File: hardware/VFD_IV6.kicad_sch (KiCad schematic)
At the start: 94 parts, among them J1 Conn_01x09, Q2 BC817, U1 4511, U10 TBD62783A, U11 4511, U12 TBD62783A, U13 4017, U2 TBD62783A, U3 4511, U4 TBD62783A, U5 4511, U6 TBD62783A, U7 4511, U8 TBD62783A, U9 4511

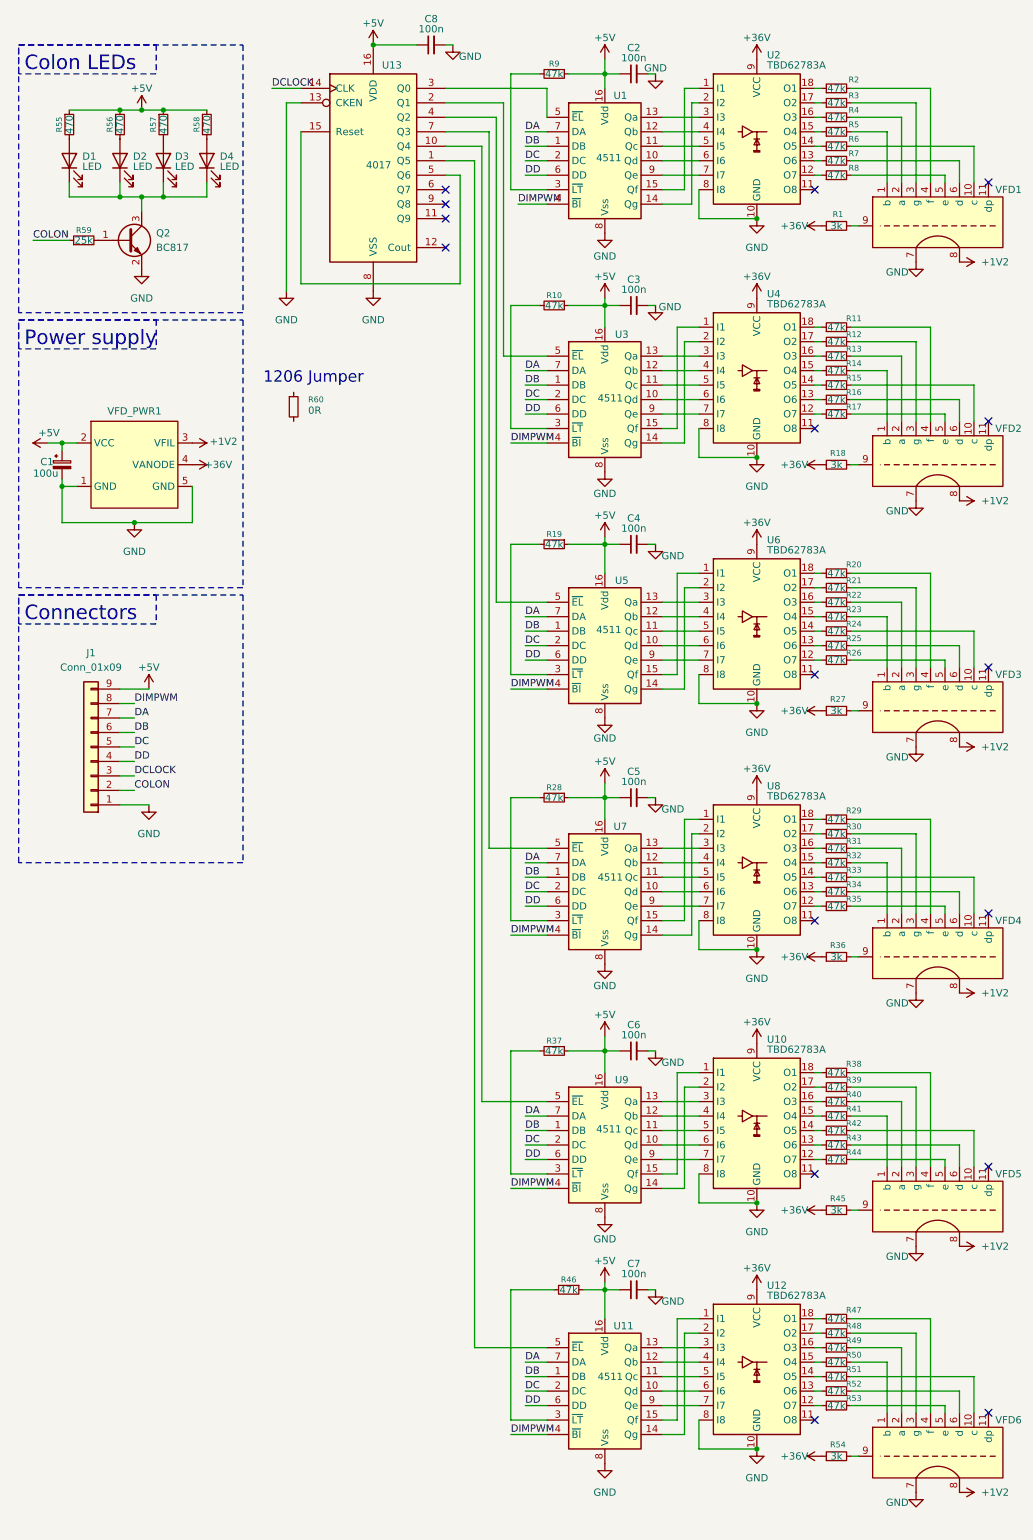
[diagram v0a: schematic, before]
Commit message: Updated schematic pdf
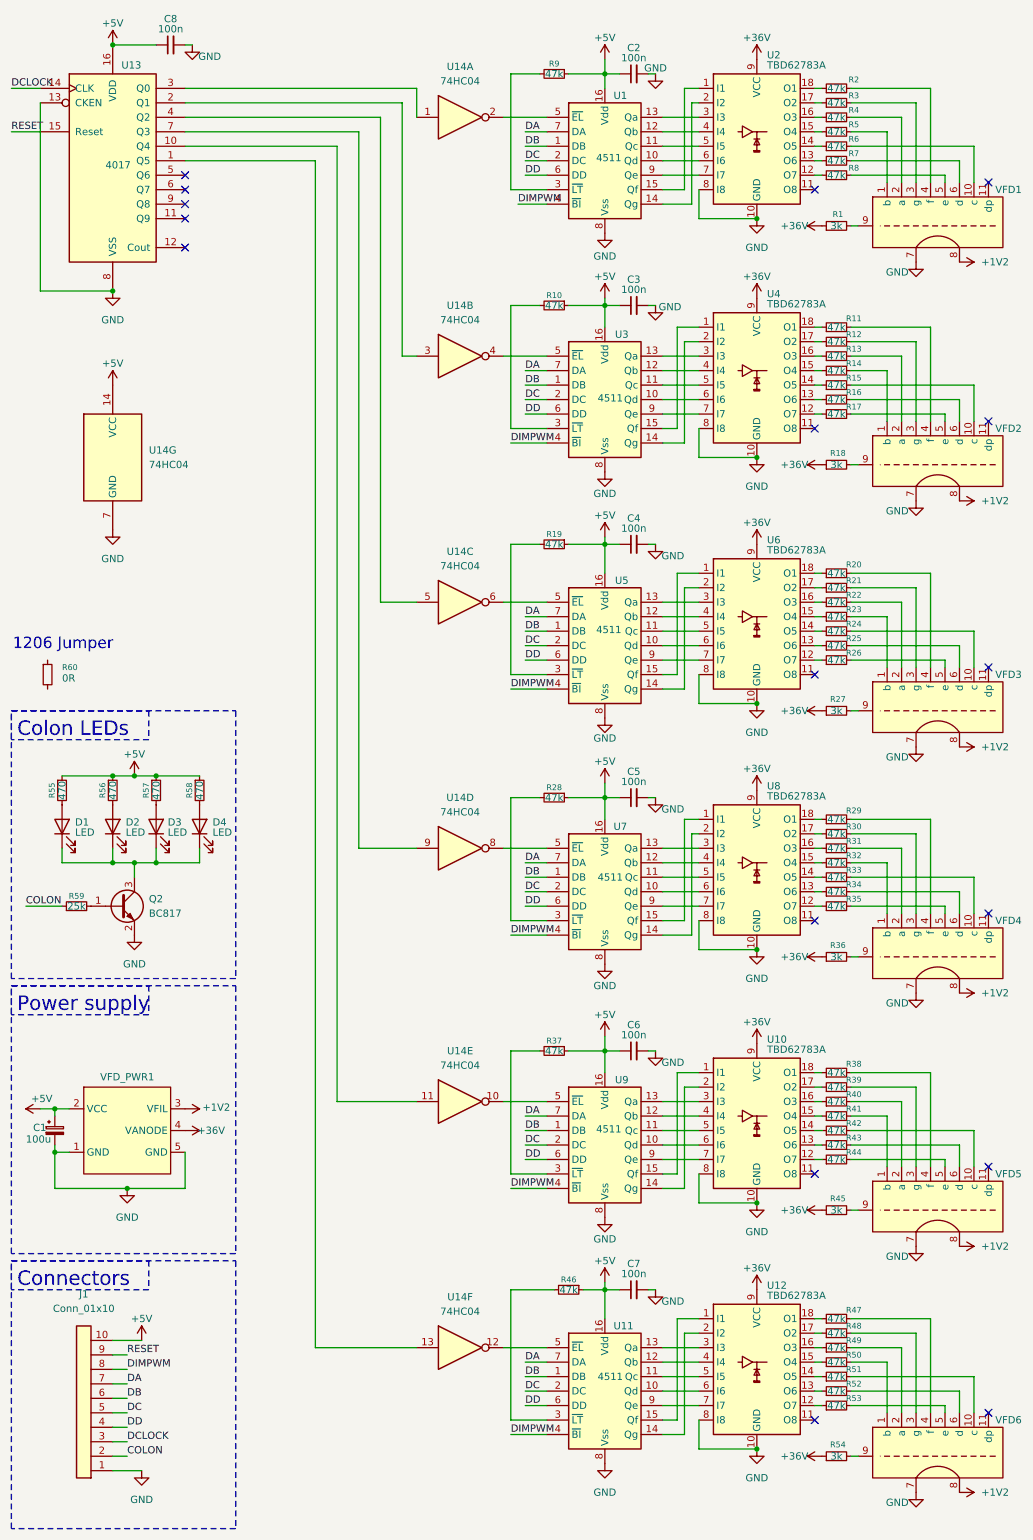
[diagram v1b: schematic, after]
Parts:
- added U14: 74HC04, Package_SO:SOIC-14_3.9x8.7mm_P1.27mm, symbol 74xx:74HC04
- J1: value Conn_01x09 -> Conn_01x10
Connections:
- net +5V: now also J1.10 (Pin_10), U14.14 (VCC); no longer J1.9 (Pin_9)
- net GND: now also U14.7 (GND)
- net at U1.5 (~{EL}): now also U14.2; no longer U13.3 (Q0)
- net at U11.5 (~{EL}): now also U14.12; no longer U13.1 (Q5)
- net at U13.10 (Q4): now also U14.11; no longer U9.5 (~{EL})
- net at U13.5 (Q6): no longer U13.15 (Reset)
- net at U13.2 (Q1): now also U14.3; no longer U3.5 (~{EL})
- net at U13.4 (Q2): now also U14.5; no longer U5.5 (~{EL})
- net at U13.7 (Q3): now also U14.9; no longer U7.5 (~{EL})
- new net: U13.1 (Q5), U14.13
- new net: U13.3 (Q0), U14.1
- new net: U14.8, U7.5 (~{EL})
- new net: U14.10, U9.5 (~{EL})
- new net: U14.6, U5.5 (~{EL})
- new net: U14.4, U3.5 (~{EL})
- new net RESET: J1.9 (Pin_9), U13.15 (Reset)
- no-connect marks 16 -> 17
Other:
- moved on the sheet: C1, C8, D1, D2, D3, D4, Q2, R55, R56, R57, R58, R59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
